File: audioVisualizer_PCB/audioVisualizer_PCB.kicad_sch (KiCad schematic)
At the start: 40 parts, among them J1 USB_C_16P, J2 SWD_DEBUG, J3 SPI_LED_MATRIX, J4 test_con, SW1 SW_Push, U1 AMS1117-3.3, U7 STM32F401CCUx, Y1 ASE-25MHz

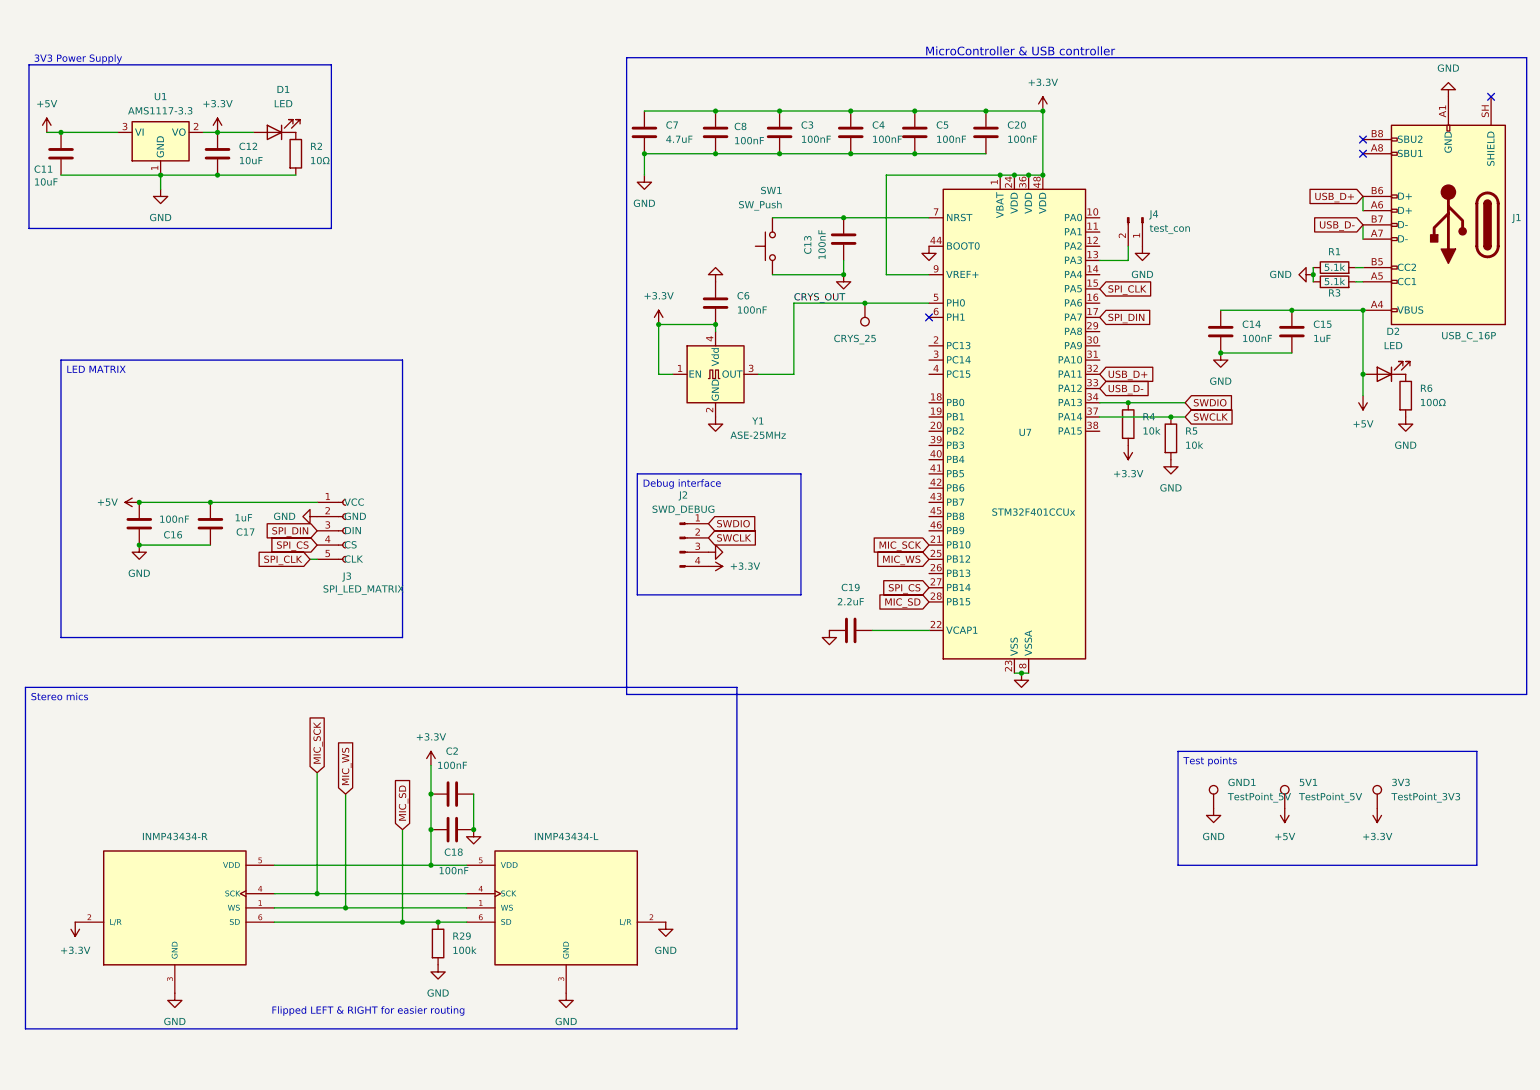
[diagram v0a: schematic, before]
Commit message: update
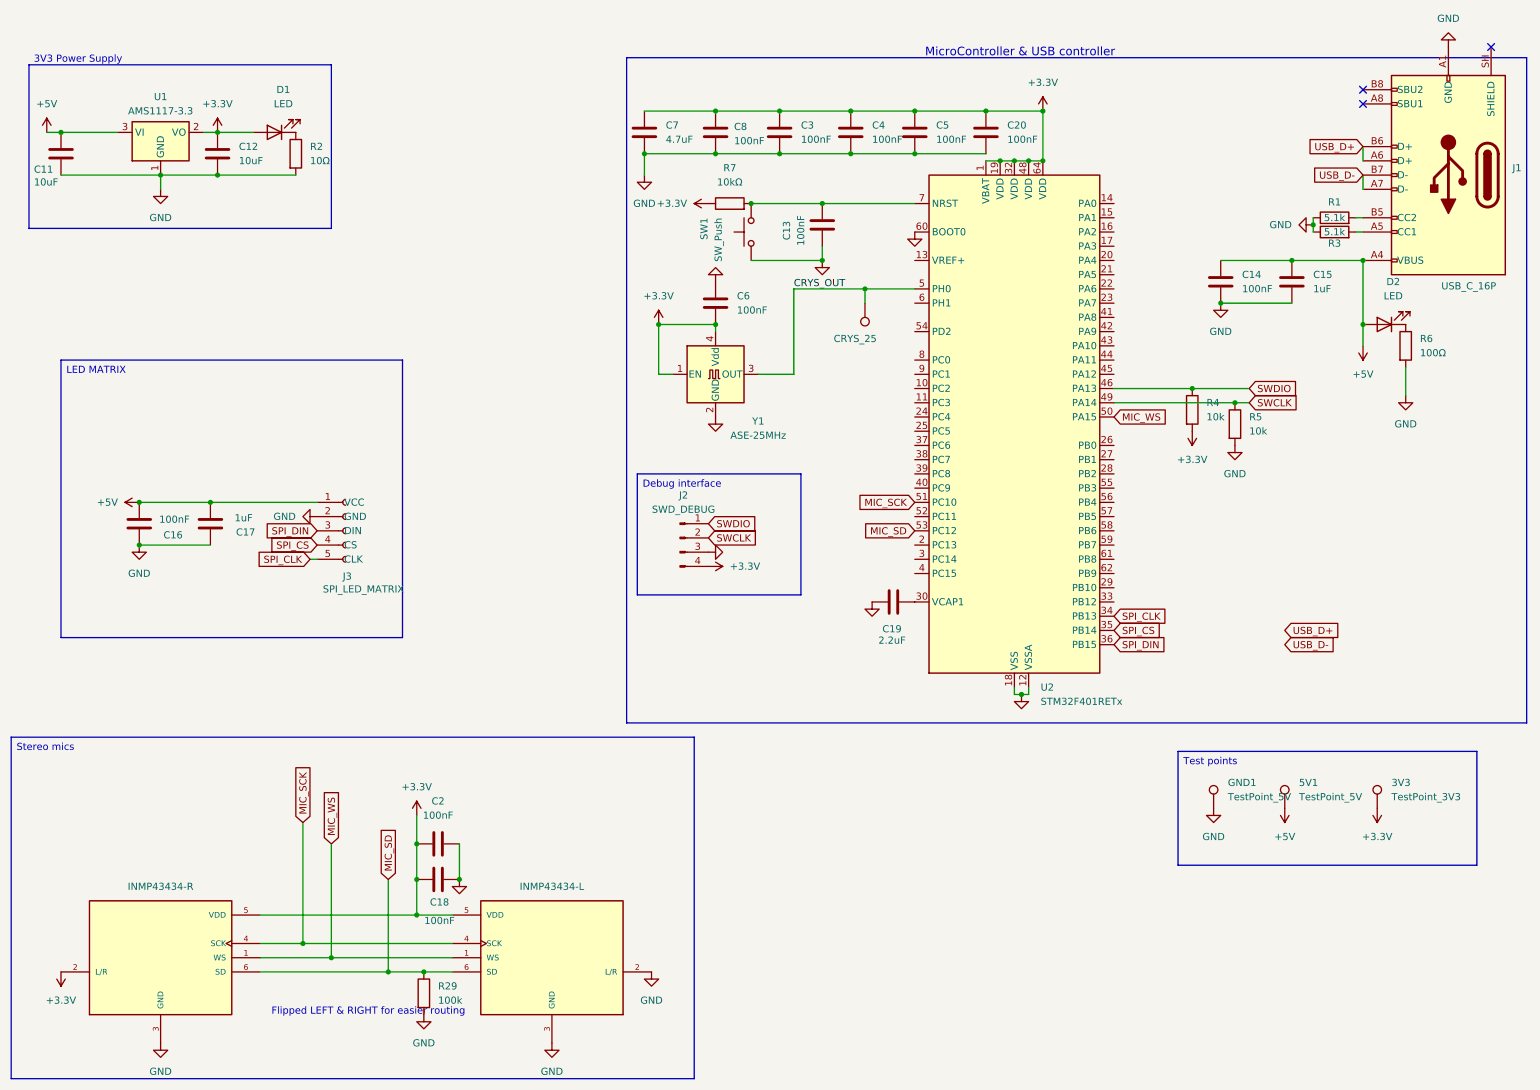
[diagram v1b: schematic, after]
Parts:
- removed J4: test_con, Connector_PinHeader_2.54mm:PinHeader_1x02_P2.54mm_Vertical, symbol Connector:Conn_01x02_Pin
- removed U7: STM32F401CCUx, Package_DFN_QFN:QFN-48-1EP_7x7mm_P0.5mm_EP5.6x5.6mm, symbol MCU_ST_STM32F4:STM32F401CCUx
- added R7: 10kΩ, Resistor_SMD:R_0805_2012Metric, symbol Device:R
- added U2: STM32F401RETx, Package_QFP:LQFP-64_10x10mm_P0.5mm, symbol MCU_ST_STM32F4:STM32F401RETx
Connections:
- net +3.3V: now also R7.1, U2.1 (VBAT), U2.19 (VDD), U2.32 (VDD), U2.48 (VDD), U2.64 (VDD)
- net CRYS_OUT: now also U2.5 (PH0)
- net GND: now also U2.12 (VSSA), U2.18 (VSS), U2.31 (VSS), U2.47 (VSS), U2.60 (BOOT0), U2.63 (VSS)
- net MIC_SCK: now also U2.51 (PC10)
- net MIC_SD: now also U2.53 (PC12)
- net MIC_WS: now also U2.50 (PA15)
- net SPI_CLK: now also U2.34 (PB13)
- net SPI_CS: now also U2.35 (PB14)
- net SPI_DIN: now also U2.36 (PB15)
- net SWCLK: now also U2.49 (PA14)
- net SWDIO: now also U2.46 (PA13)
- net at C19.1: now also U2.30 (VCAP1)
- net at C13.1, SW1.2: now also R7.2, U2.7 (NRST)
- no-connect marks 4 -> 3
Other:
- moved on the sheet: C13, C14, C15, C18, C19, C2, D2, J1, R1, R29, R3, R4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
